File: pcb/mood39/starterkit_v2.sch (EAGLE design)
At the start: 19 parts, among them IC1 TINY85, IC2 LP2950

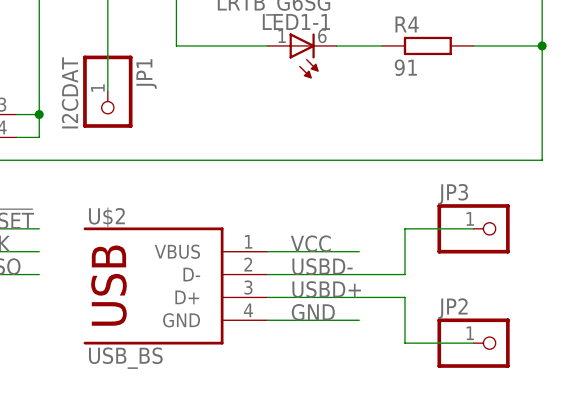
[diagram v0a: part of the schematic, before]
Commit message: start routing
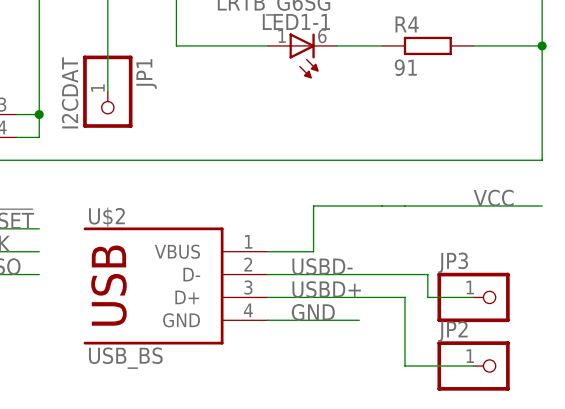
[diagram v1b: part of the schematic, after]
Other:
- moved on the sheet: JP2, JP3
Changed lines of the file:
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@@
 <instance part="S1" gate="S$1" x="73.66" y="50.8" rot="R270"/>
 <instance part="U$1" gate="G$1" x="-30.48" y="88.9" rot="R180"/>
-<instance part="JP2" gate="G$1" x="132.08" y="25.4"/>
-<instance part="JP3" gate="G$1" x="132.08" y="38.1"/>
+<instance part="JP2" gate="G$1" x="132.08" y="22.86"/>
+<instance part="JP3" gate="G$1" x="132.08" y="30.48"/>
 <instance part="U$2" gate="G$1" x="93.98" y="30.48"/>
 </instances>
@@
 </segment>
 <segment>
-<wire x1="106.68" y1="35.56" x2="116.84" y2="35.56" width="0.1524" layer="91"/>
-<label x="109.22" y="35.56" size="1.778" layer="95"/>
+<label x="129.54" y="40.64" size="1.778" layer="95"/>
+<wire x1="111.76" y1="40.64" x2="111.76" y2="35.56" width="0.1524" layer="91"/>
 <pinref part="U$2" gate="G$1" pin="VBUS"/>
+<wire x1="111.76" y1="35.56" x2="106.68" y2="35.56" width="0.1524" layer="91"/>
+<wire x1="111.76" y1="40.64" x2="119.38" y2="40.64" width="0.1524" layer="91"/>
+<wire x1="121.92" y1="40.64" x2="137.16" y2="40.64" width="0.1524" layer="91"/>
+<wire x1="121.92" y1="40.64" x2="119.38" y2="40.64" width="0.1524" layer="91"/>
 </segment>
 </net>
@@
 <net name="USBD-" class="0">
 <segment>
-<wire x1="106.68" y1="33.02" x2="121.92" y2="33.02" width="0.1524" layer="91"/>
+<wire x1="106.68" y1="33.02" x2="124.46" y2="33.02" width="0.1524" layer="91"/>
+<wire x1="124.46" y1="33.02" x2="124.46" y2="30.48" width="0.1524" layer="91"/>
+<wire x1="124.46" y1="30.48" x2="129.54" y2="30.48" width="0.1524" layer="91"/>
 <label x="109.22" y="33.02" size="1.778" layer="95"/>
 <pinref part="JP3" gate="G$1" pin="1"/>
-<wire x1="129.54" y1="38.1" x2="121.92" y2="38.1" width="0.1524" layer="91"/>
-<wire x1="121.92" y1="38.1" x2="121.92" y2="33.02" width="0.1524" layer="91"/>
 <pinref part="U$2" gate="G$1" pin="D-"/>
 </segment>
@@
 <segment>
 <wire x1="106.68" y1="30.48" x2="121.92" y2="30.48" width="0.1524" layer="91"/>
-<wire x1="121.92" y1="30.48" x2="121.92" y2="25.4" width="0.1524" layer="91"/>
-<wire x1="121.92" y1="25.4" x2="129.54" y2="25.4" width="0.1524" layer="91"/>
+<wire x1="121.92" y1="30.48" x2="121.92" y2="22.86" width="0.1524" layer="91"/>
+<wire x1="121.92" y1="22.86" x2="129.54" y2="22.86" width="0.1524" layer="91"/>
 <label x="109.22" y="30.48" size="1.778" layer="95"/>
 <pinref part="JP2" gate="G$1" pin="1"/>
